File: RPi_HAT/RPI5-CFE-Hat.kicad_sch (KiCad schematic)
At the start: 55 parts, among them J1 Conn_01x16_Shielded, J2 SFP, J3 Bus_M.2_Socket_M, J5 Conn_02x03_Odd_Even, U1 TPS564242DRLR, U2 PCA9306, U3 LM1117MP-1.8

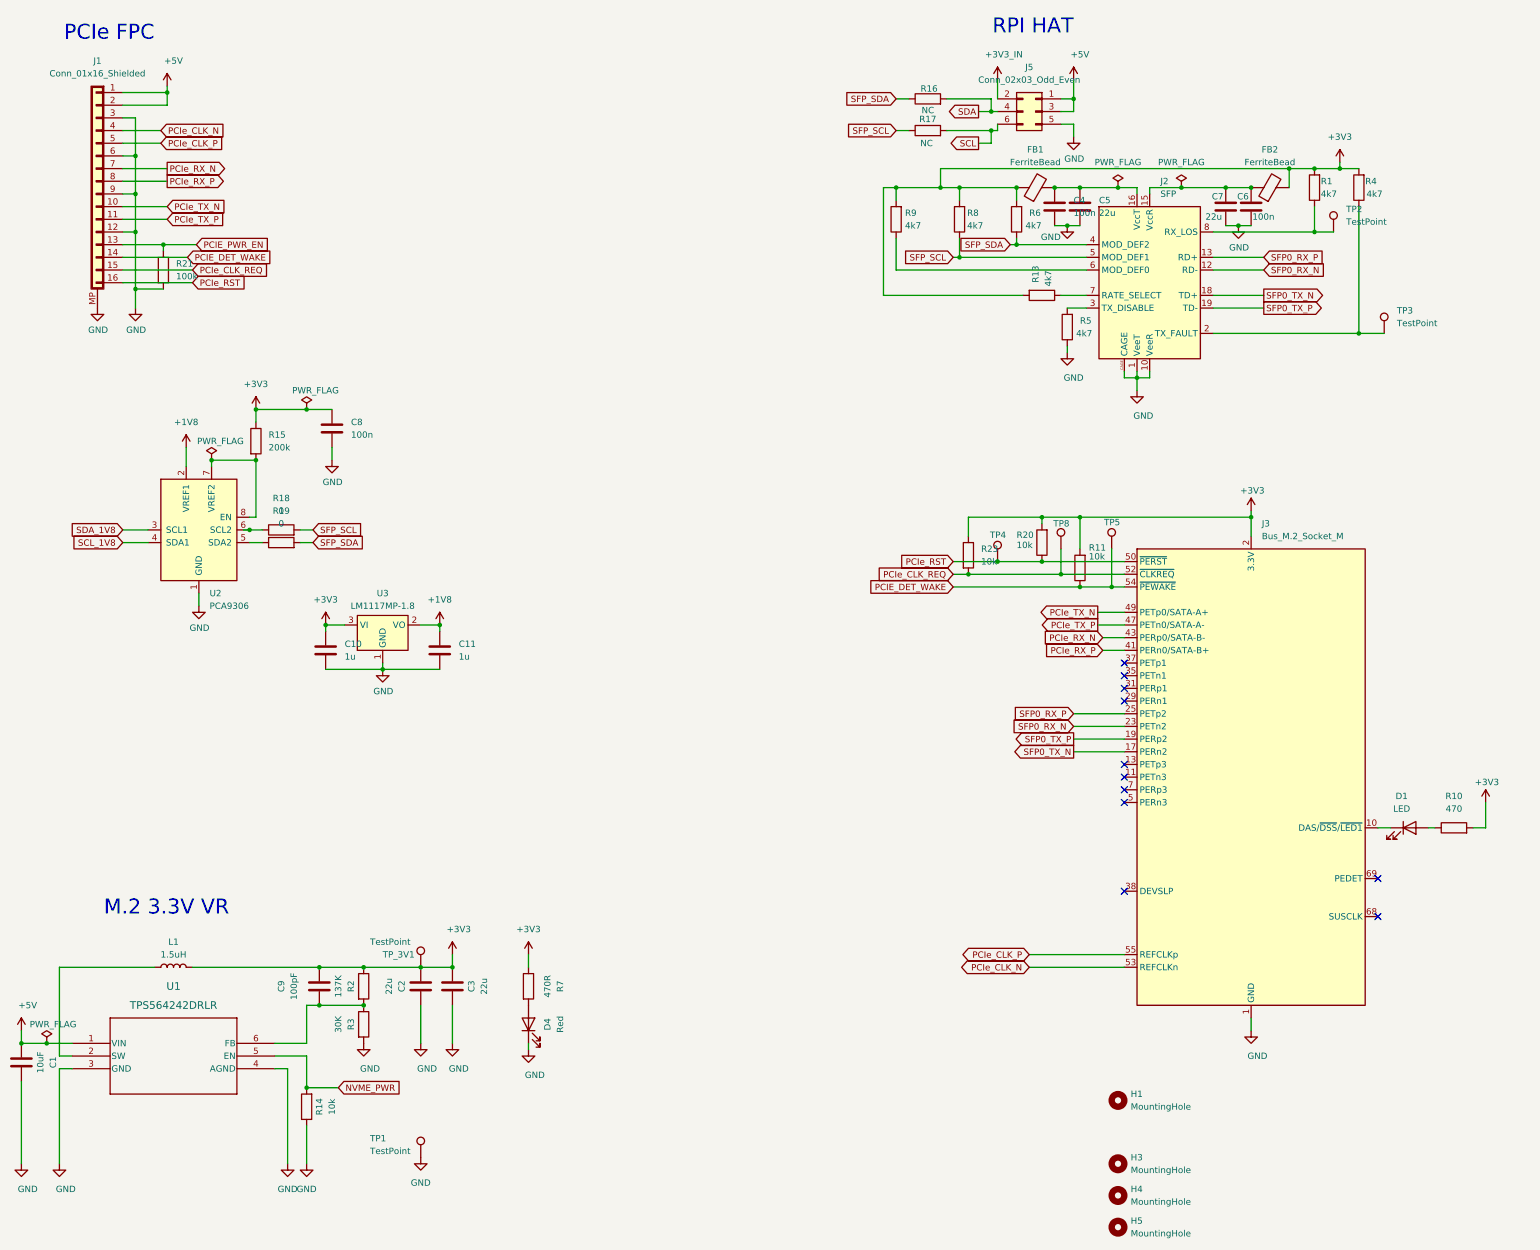
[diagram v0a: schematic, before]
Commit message: update board
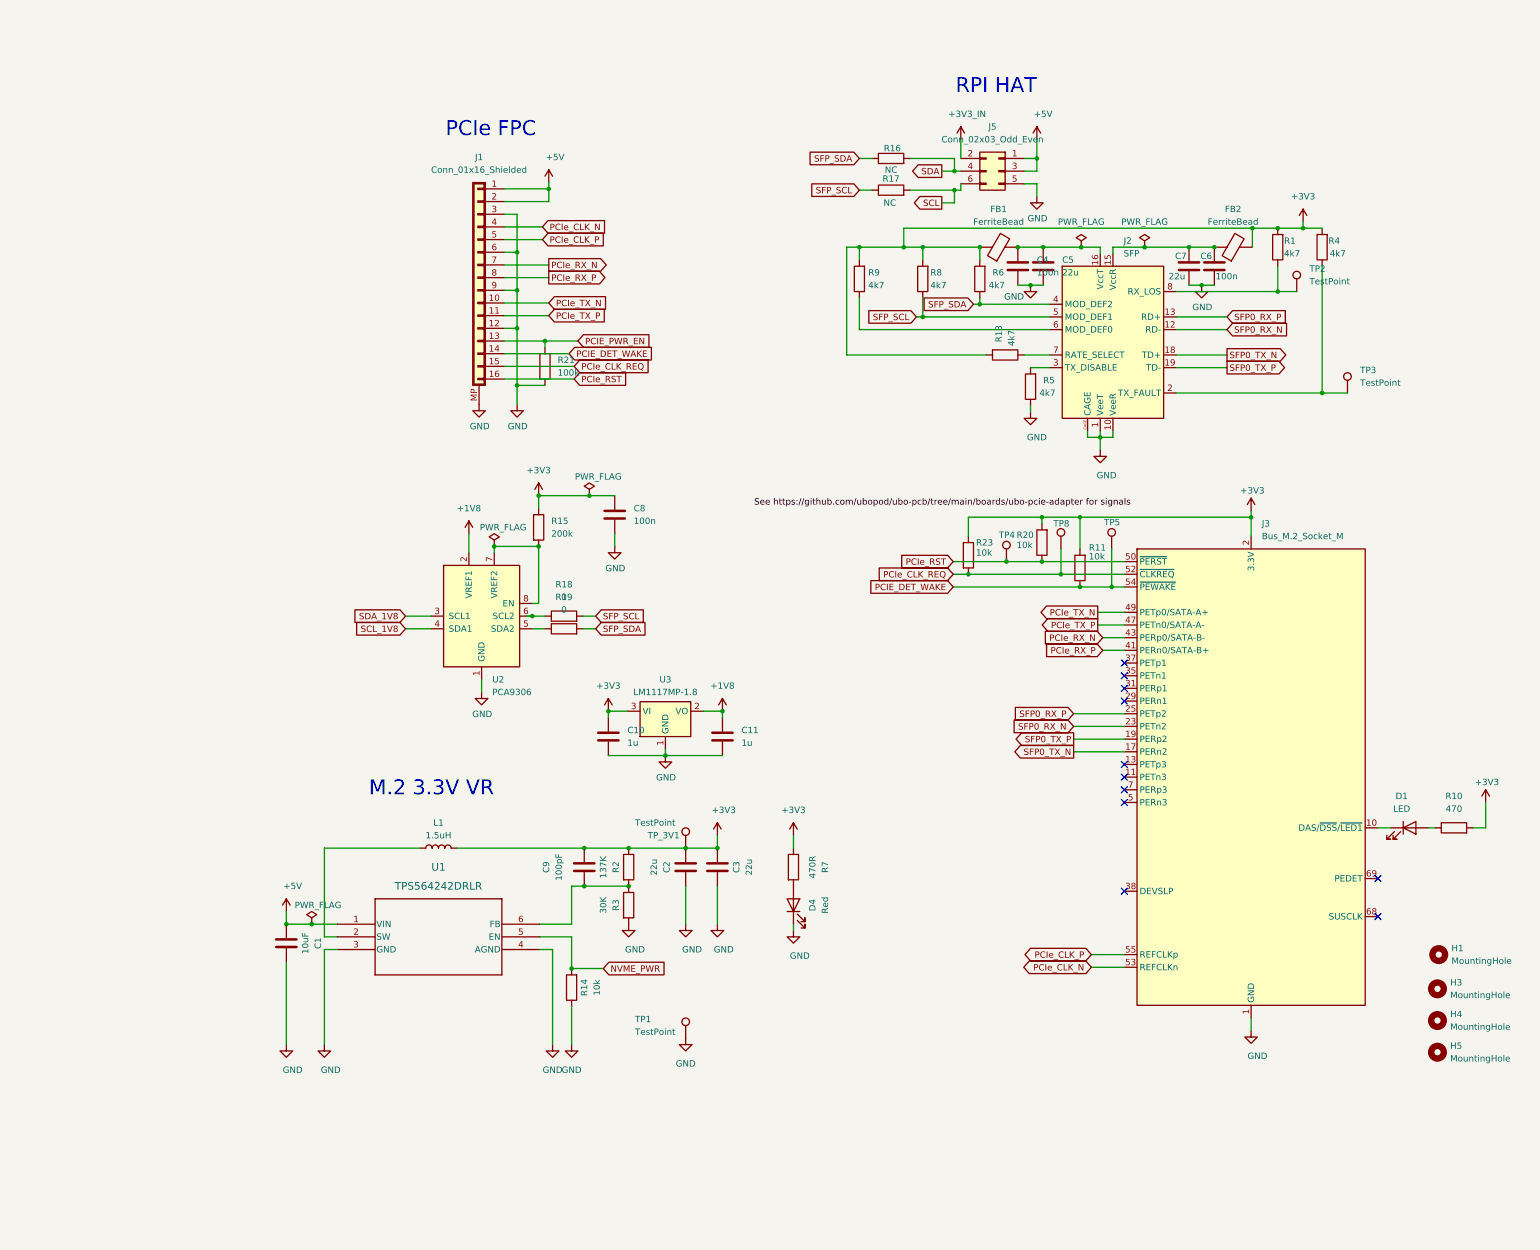
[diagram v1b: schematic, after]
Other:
- company: Will Whang -> JM Friedt
- title: RPI5-CFE-Hat -> RPI5-M2-SFP-Hat
- moved on the sheet: C1, C10, C11, C2, C3, C4, C5, C6, C7, C8, C9, D4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
